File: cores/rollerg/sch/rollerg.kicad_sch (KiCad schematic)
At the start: 1 part

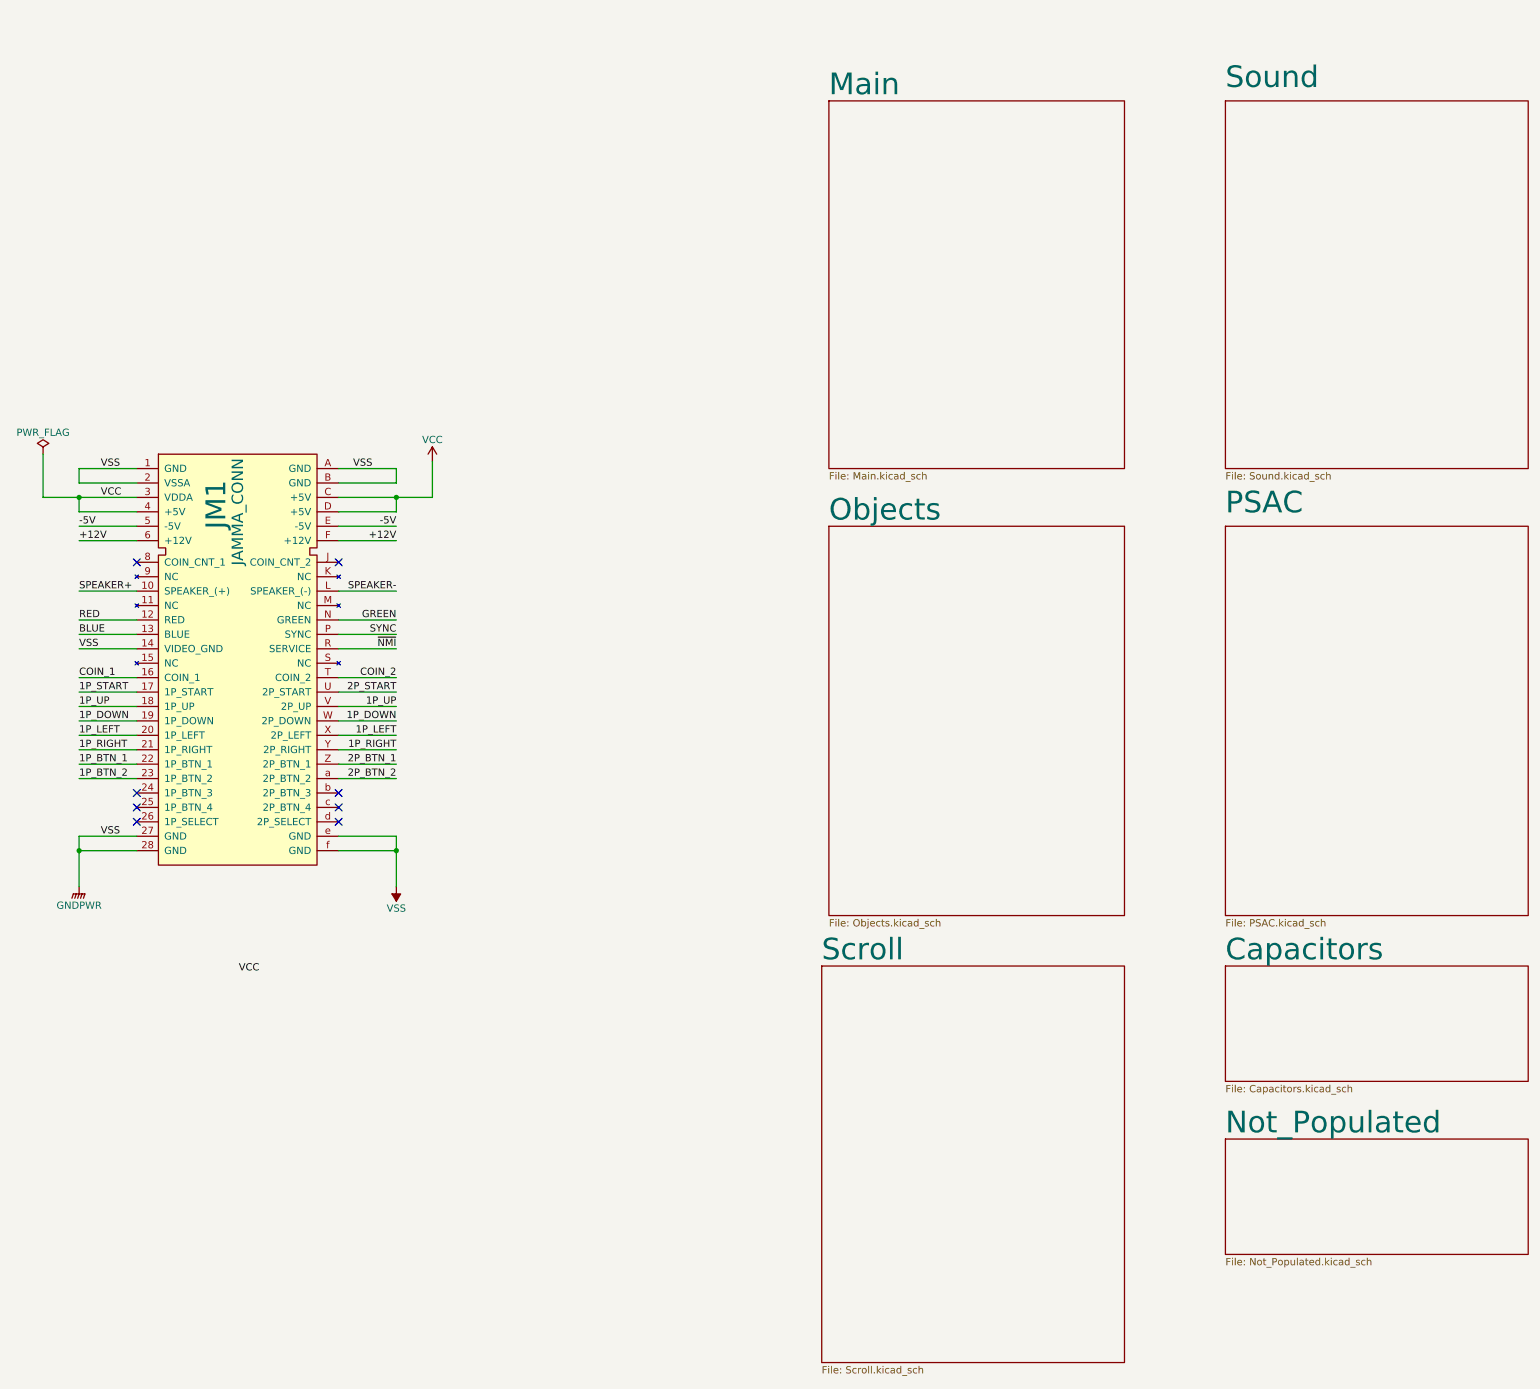
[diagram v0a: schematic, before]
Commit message: wip rollerg sch: PSAC
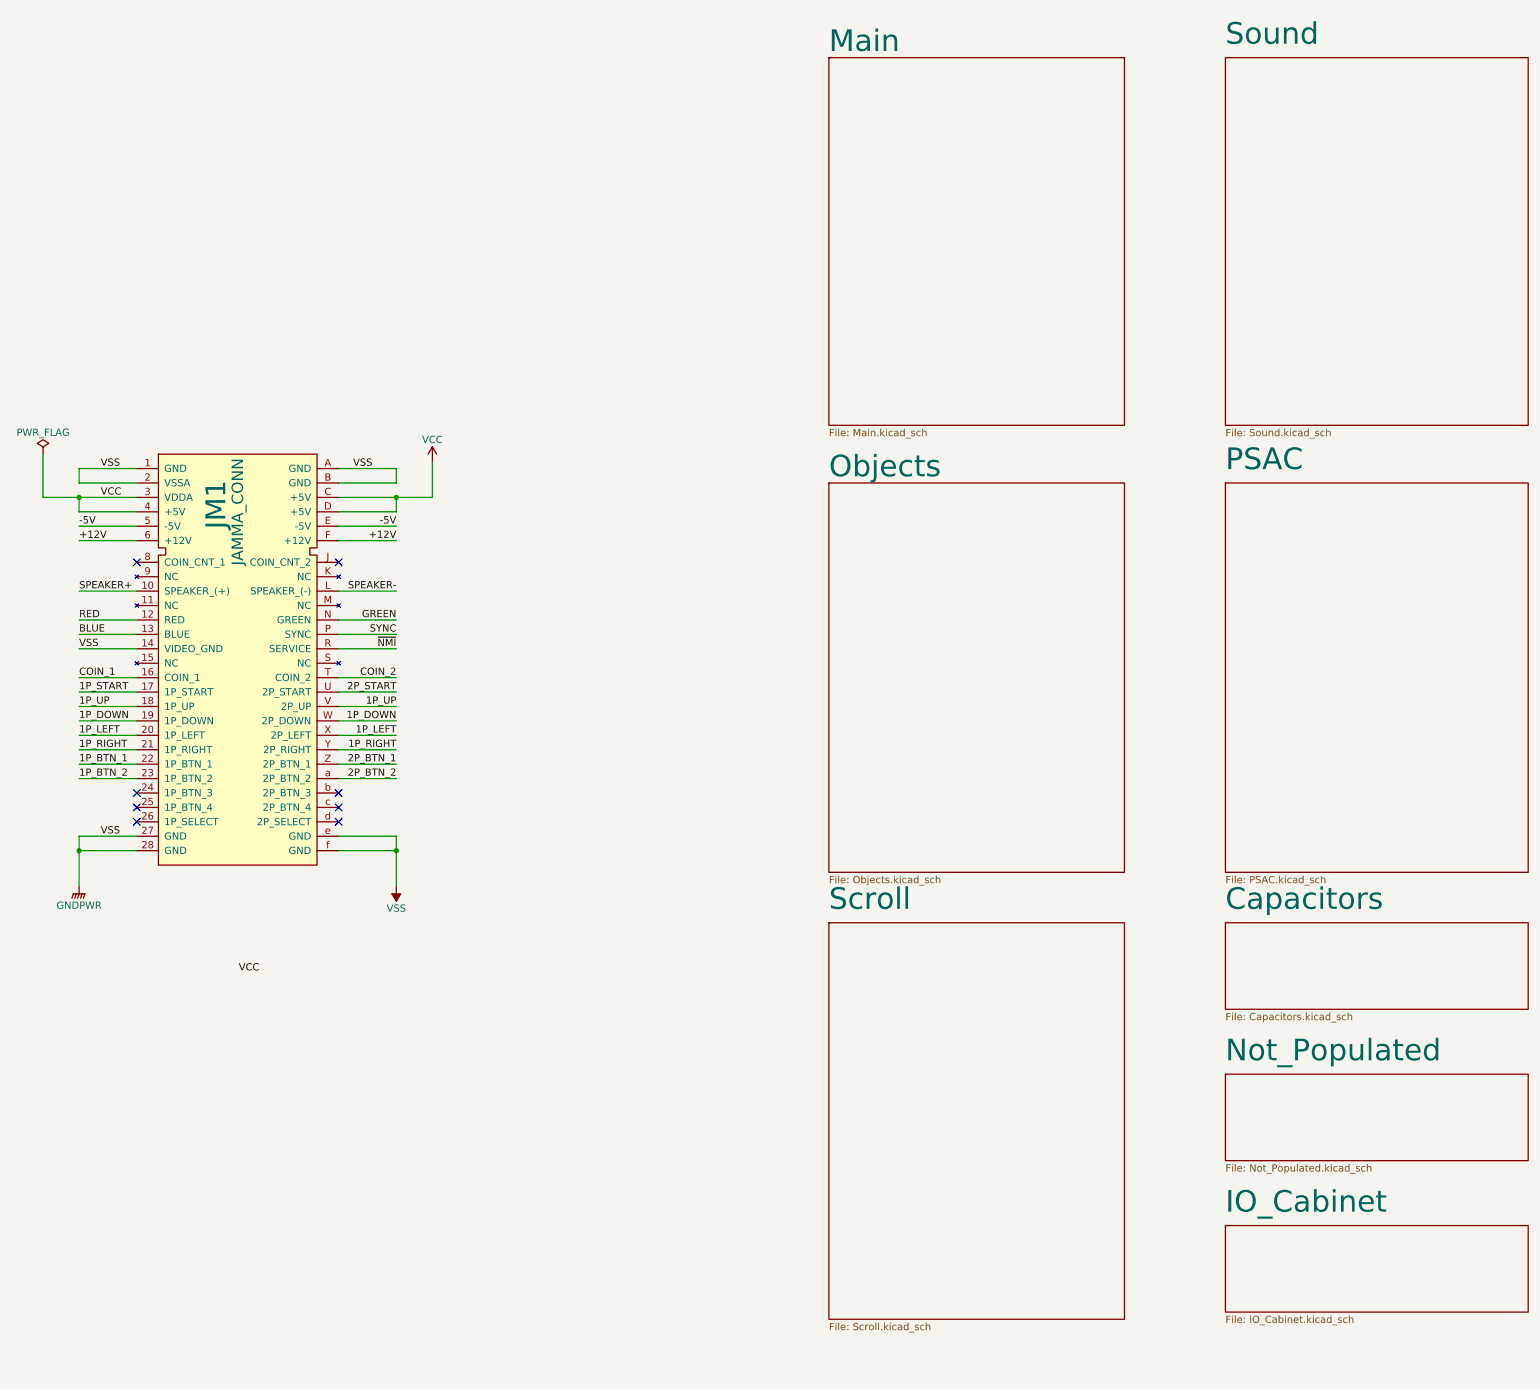
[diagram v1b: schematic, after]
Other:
- added sheet IO_Cabinet (IO_Cabinet.kicad_sch)
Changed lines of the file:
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@@
 	)
 	(sheet
-		(at 176.53 33.02)
+		(at 246.38 231.14)
+		(size 53.34 15.24)
+		(fields_autoplaced yes)
+		(stroke
+			(width 0.1524)
+			(type solid)
+		)
+		(fill
+			(color 0 0 0 0.0000)
+		)
+		(property "Sheetname" "IO_Cabinet"
+			(at 246.38 229.1584 0)
+			(effects
+				(font
+					(size 3.81 3.81)
+				)
+				(justify left bottom)
+			)
+		)
+		(property "Sheetfile" "IO_Cabinet.kicad_sch"
+			(at 246.38 246.9646 0)
+			(effects
+				(font
+					(size 1.27 1.27)
+				)
+				(justify left top)
+			)
+		)
+		(instances
+			(project "rollerg"
+				(path "/bb61a05c-9ea0-4d47-a326-1f7e835840f3"
+					(page "9")
+				)
+			)
+		)
+	)
+	(sheet
+		(at 176.53 25.4)
 		(size 52.07 64.77)
 		(fields_autoplaced yes)
@@
 		)
 		(property "Sheetname" "Main"
-			(at 176.53 32.3084 0)
+			(at 176.53 24.6884 0)
 			(effects
 				(font
@@
 		)
 		(property "Sheetfile" "Main.kicad_sch"
-			(at 176.53 98.3746 0)
+			(at 176.53 90.7546 0)
 			(effects
 				(font
@@
 	)
 	(sheet
-		(at 176.53 107.95)
+		(at 176.53 100.33)
 		(size 52.07 68.58)
 		(fields_autoplaced yes)
@@
 		)
 		(property "Sheetname" "Objects"
-			(at 176.53 107.2384 0)
+			(at 176.53 99.6184 0)
 			(effects
 				(font
@@
 		)
 		(property "Sheetfile" "Objects.kicad_sch"
-			(at 176.53 177.1146 0)
+			(at 176.53 169.4946 0)
 			(effects
 				(font
@@
 	)
 	(sheet
-		(at 246.38 107.95)
+		(at 246.38 100.33)
 		(size 53.34 68.58)
 		(fields_autoplaced yes)
@@
 		)
 		(property "Sheetname" "PSAC"
-			(at 246.38 105.9684 0)
+			(at 246.38 98.3484 0)
 			(effects
 				(font
@@
 		)
 		(property "Sheetfile" "PSAC.kicad_sch"
-			(at 246.38 177.1146 0)
+			(at 246.38 169.4946 0)
 			(effects
 				(font
@@
 	)
 	(sheet
-		(at 246.38 33.02)
+		(at 246.38 25.4)
 		(size 53.34 64.77)
 		(fields_autoplaced yes)
@@
 		)
 		(property "Sheetname" "Sound"
-			(at 246.38 31.0384 0)
+			(at 246.38 23.4184 0)
 			(effects
 				(font
@@
 		)
 		(property "Sheetfile" "Sound.kicad_sch"
-			(at 246.38 98.3746 0)
+			(at 246.38 90.7546 0)
 			(effects
 				(font
@@
 	)
 	(sheet
-		(at 246.38 185.42)
-		(size 53.34 20.32)
+		(at 246.38 177.8)
+		(size 53.34 15.24)
 		(fields_autoplaced yes)
 		(stroke
@@
 		)
 		(property "Sheetname" "Capacitors"
-			(at 246.38 184.7084 0)
+			(at 246.38 175.8184 0)
 			(effects
 				(font
@@
 		)
 		(property "Sheetfile" "Capacitors.kicad_sch"
-			(at 246.38 206.3246 0)
+			(at 246.38 193.6246 0)
 			(effects
 				(font
@@
 	)
 	(sheet
-		(at 175.26 185.42)
-		(size 53.34 69.85)
+		(at 176.53 177.8)
+		(size 52.07 69.85)
 		(fields_autoplaced yes)
 		(stroke
@@
 		)
 		(property "Sheetname" "Scroll"
-			(at 175.26 184.7084 0)
+			(at 176.53 175.8184 0)
 			(effects
 				(font
@@
 		)
 		(property "Sheetfile" "Scroll.kicad_sch"
-			(at 175.26 255.8546 0)
+			(at 176.53 248.2346 0)
 			(effects
 				(font
@@
 	)
 	(sheet
-		(at 246.38 215.9)
-		(size 53.34 20.32)
+		(at 246.38 204.47)
+		(size 53.34 15.24)
 		(fields_autoplaced yes)
 		(stroke
@@
 		)
 		(property "Sheetname" "Not_Populated"
-			(at 246.38 215.1884 0)
+			(at 246.38 202.4884 0)
 			(effects
 				(font
@@
 		)
 		(property "Sheetfile" "Not_Populated.kicad_sch"
-			(at 246.38 236.8046 0)
-			(effects
-				(font
+			(at 246.38 220.2946 0)
+			(effects
+				(font
